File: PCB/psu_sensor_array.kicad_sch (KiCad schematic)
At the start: 3 parts, among them U16 MCP9700AT-ELT, U17 MCP9700AT-ELT, U18 MCP9700AT-ELT

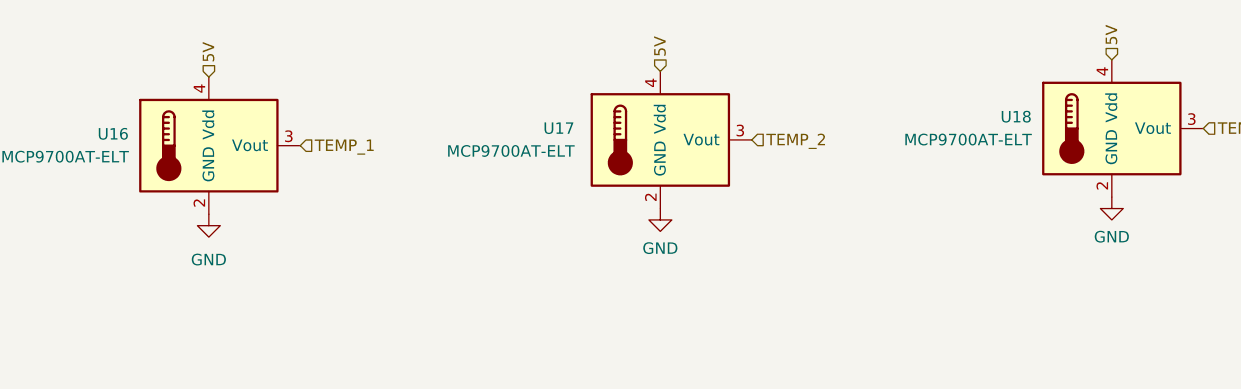
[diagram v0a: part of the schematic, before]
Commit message: v2!
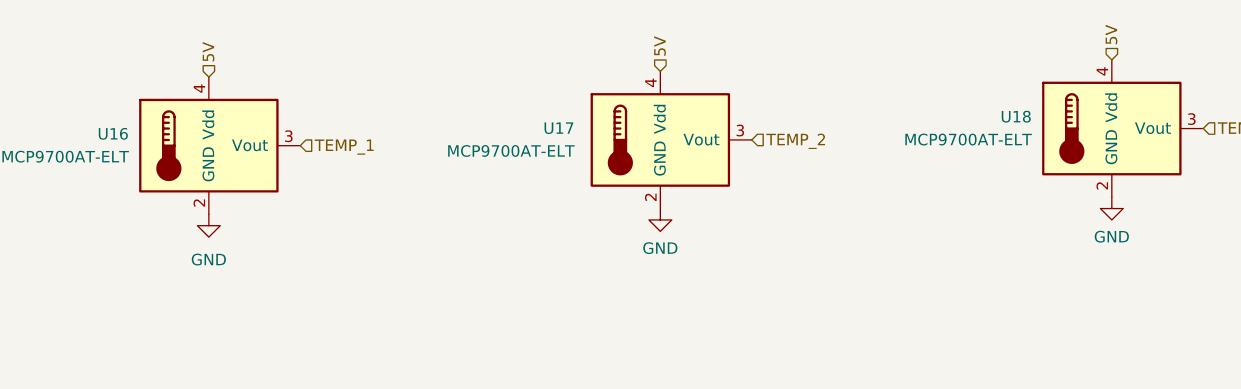
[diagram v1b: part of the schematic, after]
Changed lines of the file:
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@@
-(kicad_sch (version 20211123) (generator eeschema)
+(kicad_sch (version 20230121) (generator eeschema)
   (paper "A4")
   (title_block
@@
     (effects (font (size 1.27 1.27)) (justify left bottom))
   )
-  (hierarchical_label "TEMP_3" (shape input) (at 210.185 96.52 0)
+  (hierarchical_label "TEMP_3" (shape input) (at 210.185 96.52 0) (fields_autoplaced)
     (effects (font (size 1.27 1.27)) (justify left))
   )
-  (hierarchical_label "5V" (shape input) (at 99.695 90.805 90)
+  (hierarchical_label "5V" (shape input) (at 99.695 90.805 90) (fields_autoplaced)
     (effects (font (size 1.27 1.27)) (justify left))
   )
-  (hierarchical_label "TEMP_1" (shape input) (at 109.855 98.425 0)
+  (hierarchical_label "TEMP_1" (shape input) (at 109.855 98.425 0) (fields_autoplaced)
     (effects (font (size 1.27 1.27)) (justify left))
   )
-  (hierarchical_label "TEMP_2" (shape input) (at 160.02 97.79 0)
+  (hierarchical_label "TEMP_2" (shape input) (at 160.02 97.79 0) (fields_autoplaced)
     (effects (font (size 1.27 1.27)) (justify left))
   )
-  (hierarchical_label "5V" (shape input) (at 149.86 90.17 90)
+  (hierarchical_label "5V" (shape input) (at 149.86 90.17 90) (fields_autoplaced)
     (effects (font (size 1.27 1.27)) (justify left))
   )
-  (hierarchical_label "5V" (shape input) (at 200.025 88.9 90)
+  (hierarchical_label "5V" (shape input) (at 200.025 88.9 90) (fields_autoplaced)
     (effects (font (size 1.27 1.27)) (justify left))
   )
   (symbol (lib_id "power:GND") (at 149.86 105.41 0) (unit 1)
-    (in_bom yes) (on_board yes) (fields_autoplaced)
-    (property "Reference" "#PWR0114" (id 0) (at 149.86 111.76 0)
+    (in_bom yes) (on_board yes) (dnp no) (fields_autoplaced)
+    (property "Reference" "#PWR0114" (at 149.86 111.76 0)
       (effects (font (size 1.27 1.27)) hide)
     )
-    (property "Value" "GND" (id 1) (at 149.86 109.855 0))
-    (property "Footprint" "" (id 2) (at 149.86 105.41 0)
+    (property "Value" "GND" (at 149.86 109.855 0)
+      (effects (font (size 1.27 1.27)))
+    )
+    (property "Footprint" "" (at 149.86 105.41 0)
       (effects (font (size 1.27 1.27)) hide)
     )
-    (property "Datasheet" "" (id 3) (at 149.86 105.41 0)
+    (property "Datasheet" "" (at 149.86 105.41 0)
       (effects (font (size 1.27 1.27)) hide)
     )
     (pin "1")
+    (instances
+      (project "marvin_fc_board"
+        (path "/e63e39d7-6ac0-4ffd-8aa3-1841a4541b55/9afb9b8b-5318-4efd-b376-586a01a52ed4/7eba4d57-cdbe-4c27-a88c-4e498e96a137"
+          (reference "#PWR0114") (unit 1)
+        )
+      )
+    )
   )
   (symbol (lib_id "Sensor_Temperature:MCP9700AT-ELT") (at 99.695 98.425 0) (unit 1)
-    (in_bom yes) (on_board yes) (fields_autoplaced)
-    (property "Reference" "U16" (id 0) (at 90.805 97.1549 0)
+    (in_bom yes) (on_board yes) (dnp no) (fields_autoplaced)
+    (property "Reference" "U16" (at 90.805 97.1549 0)
       (effects (font (size 1.27 1.27)) (justify right))
     )
-    (property "Value" "MCP9700AT-ELT" (id 1) (at 90.805 99.6949 0)
+    (property "Value" "MCP9700AT-ELT" (at 90.805 99.6949 0)
       (effects (font (size 1.27 1.27)) (justify right))
     )
-    (property "Footprint" "Package_TO_SOT_SMD:SOT-353_SC-70-5" (id 2) (at 99.695 108.585 0)
+    (property "Footprint" "Package_TO_SOT_SMD:SOT-353_SC-70-5" (at 99.695 108.585 0)
       (effects (font (size 1.27 1.27)) hide)
     )
-    (property "Datasheet" "http://ww1.microchip.com/downloads/en/DeviceDoc/20001942G.pdf" (id 3) (at 99.695 98.425 0)
+    (property "Datasheet" "http://ww1.microchip.com/downloads/en/DeviceDoc/20001942G.pdf" (at 99.695 98.425 0)
       (effects (font (size 1.27 1.27)) hide)
     )
@@
     (pin "4")
     (pin "5")
+    (instances
+      (project "marvin_fc_board"
+        (path "/e63e39d7-6ac0-4ffd-8aa3-1841a4541b55/9afb9b8b-5318-4efd-b376-586a01a52ed4/7eba4d57-cdbe-4c27-a88c-4e498e96a137"
+          (reference "U16") (unit 1)
+        )
+      )
+    )
   )
   (symbol (lib_id "Sensor_Temperature:MCP9700AT-ELT") (at 200.025 96.52 0) (unit 1)
-    (in_bom yes) (on_board yes) (fields_autoplaced)
-    (property "Reference" "U18" (id 0) (at 191.135 95.2499 0)
+    (in_bom yes) (on_board yes) (dnp no) (fields_autoplaced)
+    (property "Reference" "U18" (at 191.135 95.2499 0)
       (effects (font (size 1.27 1.27)) (justify right))
     )
-    (property "Value" "MCP9700AT-ELT" (id 1) (at 191.135 97.7899 0)
+    (property "Value" "MCP9700AT-ELT" (at 191.135 97.7899 0)
       (effects (font (size 1.27 1.27)) (justify right))
     )
-    (property "Footprint" "Package_TO_SOT_SMD:SOT-353_SC-70-5" (id 2) (at 200.025 106.68 0)
+    (property "Footprint" "Package_TO_SOT_SMD:SOT-353_SC-70-5" (at 200.025 106.68 0)
       (effects (font (size 1.27 1.27)) hide)
     )
-    (property "Datasheet" "http://ww1.microchip.com/downloads/en/DeviceDoc/20001942G.pdf" (id 3) (at 200.025 96.52 0)
+    (property "Datasheet" "http://ww1.microchip.com/downloads/en/DeviceDoc/20001942G.pdf" (at 200.025 96.52 0)
       (effects (font (size 1.27 1.27)) hide)
     )
@@
     (pin "4")
     (pin "5")
+    (instances
+      (project "marvin_fc_board"
+        (path "/e63e39d7-6ac0-4ffd-8aa3-1841a4541b55/9afb9b8b-5318-4efd-b376-586a01a52ed4/7eba4d57-cdbe-4c27-a88c-4e498e96a137"
+          (reference "U18") (unit 1)
+        )
+      )
+    )
   )
   (symbol (lib_id "power:GND") (at 200.025 104.14 0) (unit 1)
-    (in_bom yes) (on_board yes) (fields_autoplaced)
-    (property "Reference" "#PWR0115" (id 0) (at 200.025 110.49 0)
+    (in_bom yes) (on_board yes) (dnp no) (fields_autoplaced)
+    (property "Reference" "#PWR0115" (at 200.025 110.49 0)
       (effects (font (size 1.27 1.27)) hide)
     )
-    (property "Value" "GND" (id 1) (at 200.025 108.585 0))
-    (property "Footprint" "" (id 2) (at 200.025 104.14 0)
+    (property "Value" "GND" (at 200.025 108.585 0)
+      (effects (font (size 1.27 1.27)))
+    )
+    (property "Footprint" "" (at 200.025 104.14 0)
       (effects (font (size 1.27 1.27)) hide)
     )
-    (property "Datasheet" "" (id 3) (at 200.025 104.14 0)
+    (property "Datasheet" "" (at 200.025 104.14 0)
       (effects (font (size 1.27 1.27)) hide)
     )
     (pin "1")
+    (instances
+      (project "marvin_fc_board"
+        (path "/e63e39d7-6ac0-4ffd-8aa3-1841a4541b55/9afb9b8b-5318-4efd-b376-586a01a52ed4/7eba4d57-cdbe-4c27-a88c-4e498e96a137"
+          (reference "#PWR0115") (unit 1)
+        )
+      )
+    )
   )
   (symbol (lib_id "power:GND") (at 99.695 106.045 0) (unit 1)
-    (in_bom yes) (on_board yes) (fields_autoplaced)
-    (property "Reference" "#PWR0113" (id 0) (at 99.695 112.395 0)
+    (in_bom yes) (on_board yes) (dnp no) (fields_autoplaced)
+    (property "Reference" "#PWR0113" (at 99.695 112.395 0)
       (effects (font (size 1.27 1.27)) hide)
     )
-    (property "Value" "GND" (id 1) (at 99.695 111.125 0))
-    (property "Footprint" "" (id 2) (at 99.695 106.045 0)
+    (property "Value" "GND" (at 99.695 111.125 0)
+      (effects (font (size 1.27 1.27)))
+    )
+    (property "Footprint" "" (at 99.695 106.045 0)
       (effects (font (size 1.27 1.27)) hide)
     )
-    (property "Datasheet" "" (id 3) (at 99.695 106.045 0)
+    (property "Datasheet" "" (at 99.695 106.045 0)
       (effects (font (size 1.27 1.27)) hide)
     )
     (pin "1")
+    (instances
+      (project "marvin_fc_board"
+        (path "/e63e39d7-6ac0-4ffd-8aa3-1841a4541b55/9afb9b8b-5318-4efd-b376-586a01a52ed4/7eba4d57-cdbe-4c27-a88c-4e498e96a137"
+          (reference "#PWR0113") (unit 1)
+        )
+      )
+    )
   )
   (symbol (lib_id "Sensor_Temperature:MCP9700AT-ELT") (at 149.86 97.79 0) (unit 1)
-    (in_bom yes) (on_board yes) (fields_autoplaced)
-    (property "Reference" "U17" (id 0) (at 140.335 96.5199 0)
+    (in_bom yes) (on_board yes) (dnp no) (fields_autoplaced)
+    (property "Reference" "U17" (at 140.335 96.5199 0)
       (effects (font (size 1.27 1.27)) (justify right))
     )
-    (property "Value" "MCP9700AT-ELT" (id 1) (at 140.335 99.0599 0)
+    (property "Value" "MCP9700AT-ELT" (at 140.335 99.0599 0)
       (effects (font (size 1.27 1.27)) (justify right))
     )
-    (property "Footprint" "Package_TO_SOT_SMD:SOT-353_SC-70-5" (id 2) (at 149.86 107.95 0)
+    (property "Footprint" "Package_TO_SOT_SMD:SOT-353_SC-70-5" (at 149.86 107.95 0)
       (effects (font (size 1.27 1.27)) hide)
     )
-    (property "Datasheet" "http://ww1.microchip.com/downloads/en/DeviceDoc/20001942G.pdf" (id 3) (at 149.86 97.79 0)
+    (property "Datasheet" "http://ww1.microchip.com/downloads/en/DeviceDoc/20001942G.pdf" (at 149.86 97.79 0)
       (effects (font (size 1.27 1.27)) hide)
     )
@@
     (pin "4")
     (pin "5")
+    (instances
+      (project "marvin_fc_board"
+        (path "/e63e39d7-6ac0-4ffd-8aa3-1841a4541b55/9afb9b8b-5318-4efd-b376-586a01a52ed4/7eba4d57-cdbe-4c27-a88c-4e498e96a137"
+          (reference "U17") (unit 1)
+        )
+      )
+    )
   )
 )
